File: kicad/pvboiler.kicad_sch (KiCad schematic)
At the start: 32 parts, among them J1 Conn_01x04, J2 Screw_Terminal_01x04, J3 Conn_01x04, J4 Screw_Terminal_01x03, U1 MOC3021M, U2 H11AA1, U3 IRM-03-5

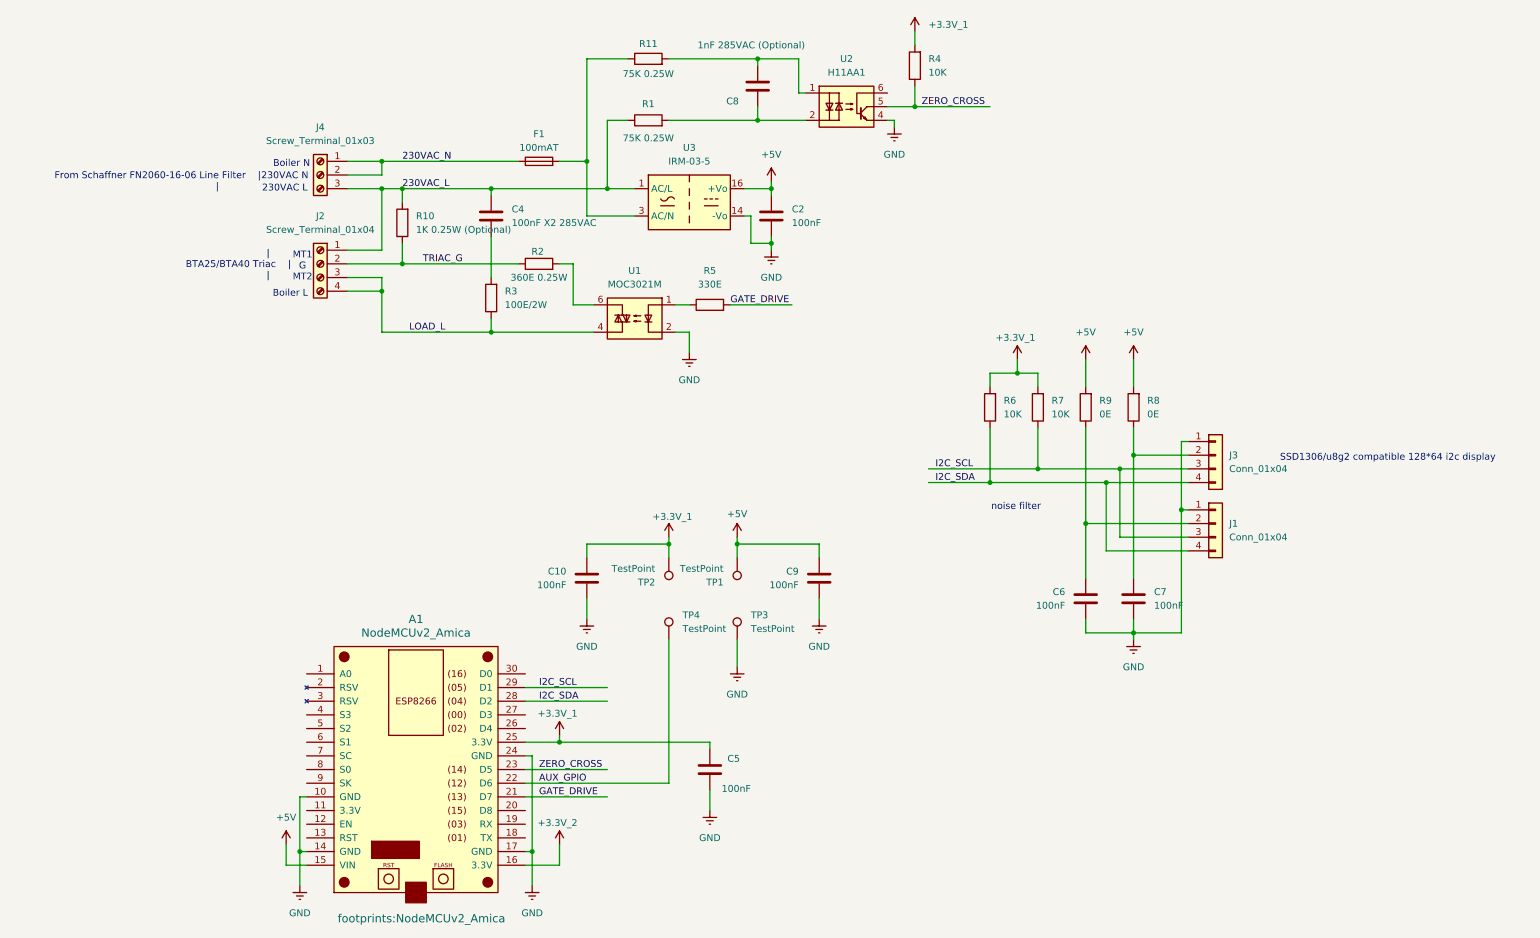
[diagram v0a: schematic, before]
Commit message: added: Schematic pdf added: Pictures
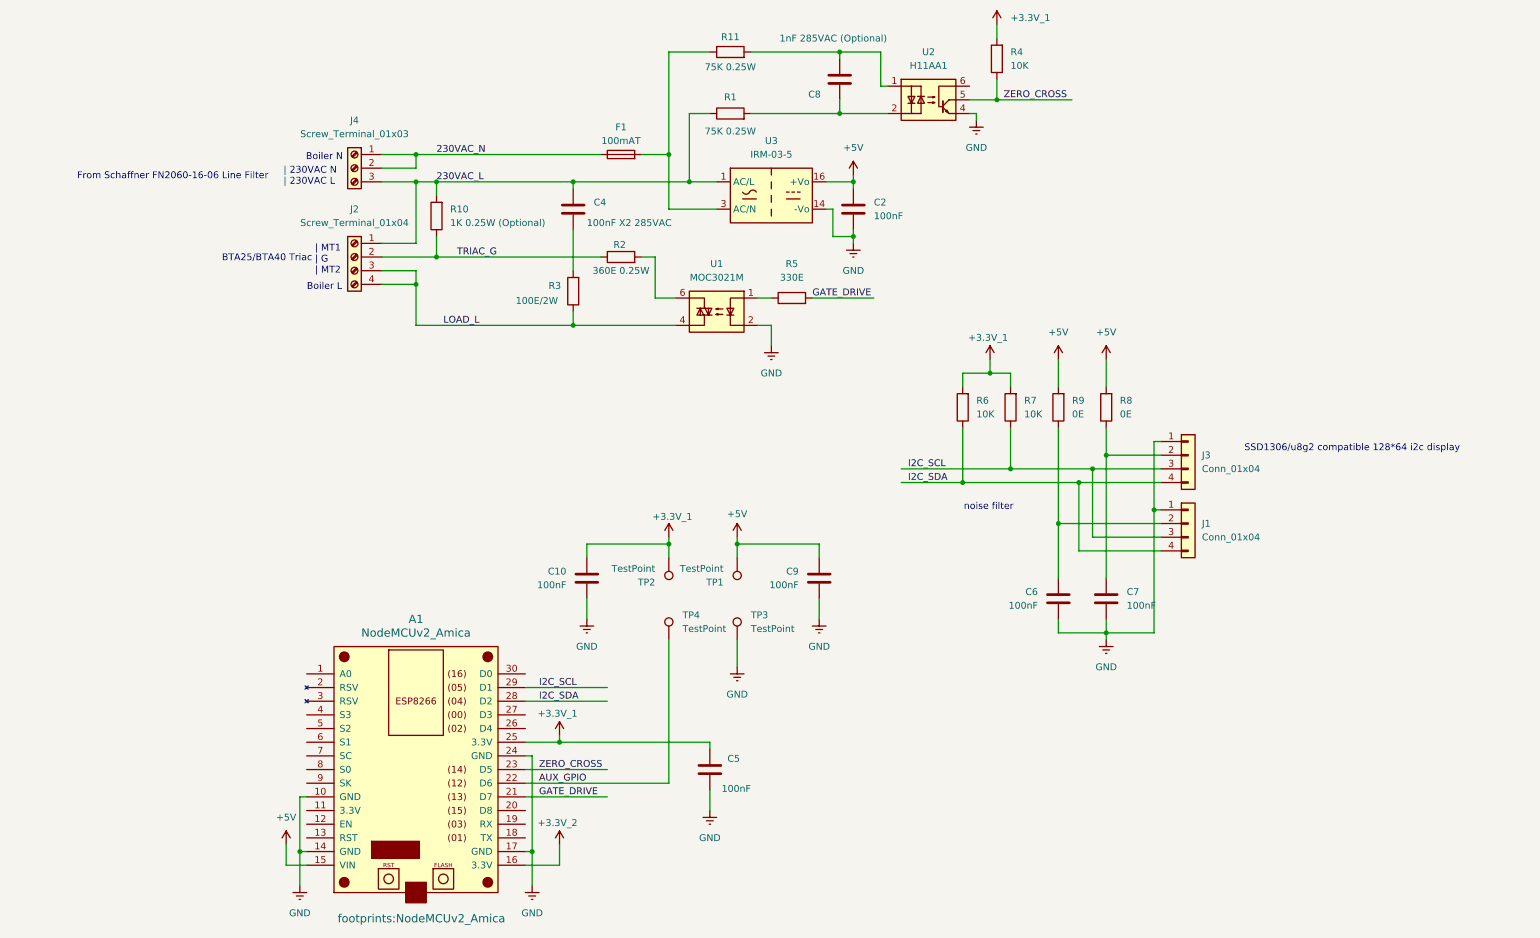
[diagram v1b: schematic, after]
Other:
- note added: "BTA25/BTA40 Triac"
- note added: "From Schaffner FN2060-16-06 Line Filter"
- note added: "| 230VAC N | 230VAC L"
- note added: "| MT1 | G | MT2"
- note removed: "230VAC L"
- note removed: "230VAC N"
- note removed: "From Schaffner FN2060-16-06 Line Filter | |"
- note removed: "MT1 G MT2"
- note removed: "| BTA25/BTA40 Triac | |"
- moved on the sheet: C2, C4, C6, C7, C8, F1, J1, J2, J3, J4, R1, R10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
